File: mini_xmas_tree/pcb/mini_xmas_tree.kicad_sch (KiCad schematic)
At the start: 19 parts, among them J1 Conn_01x02, J2 Conn_01x02, J3 Conn_01x02, J4 Conn_01x02, Q1 BC817, Q2 BC817, Q3 BC817, Q4 BC817

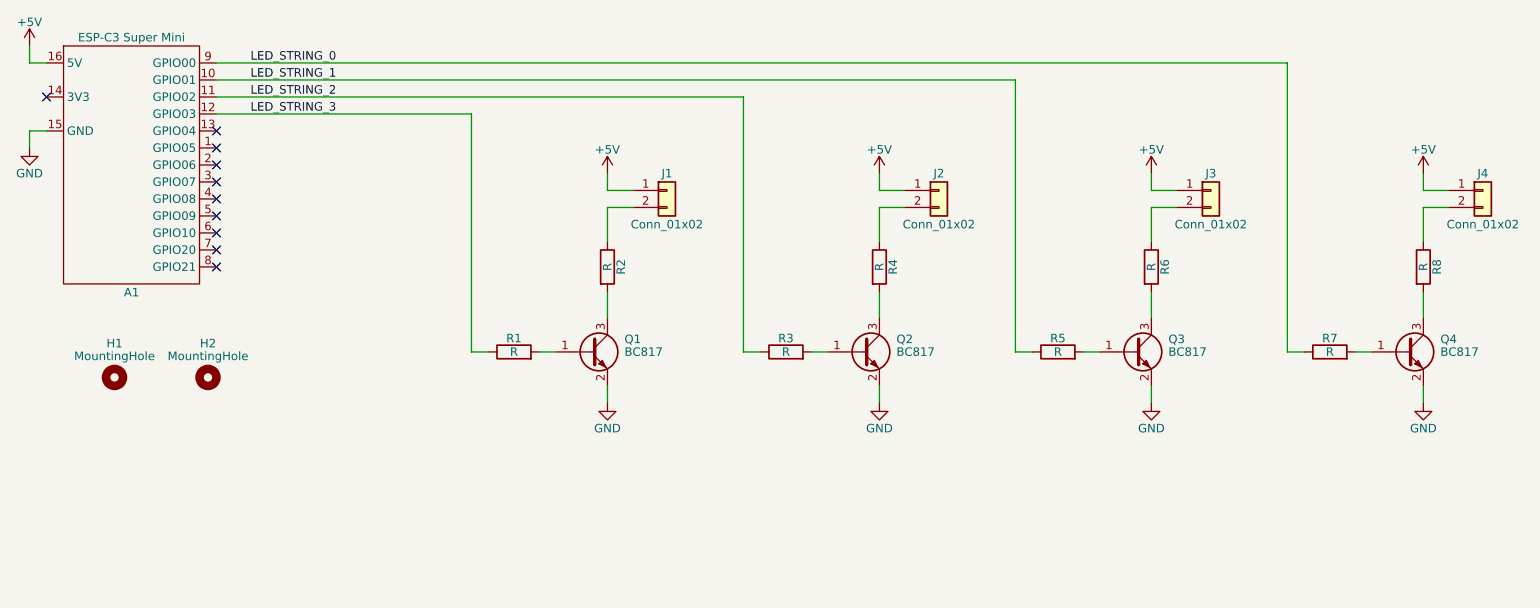
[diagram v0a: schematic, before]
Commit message: create gcode
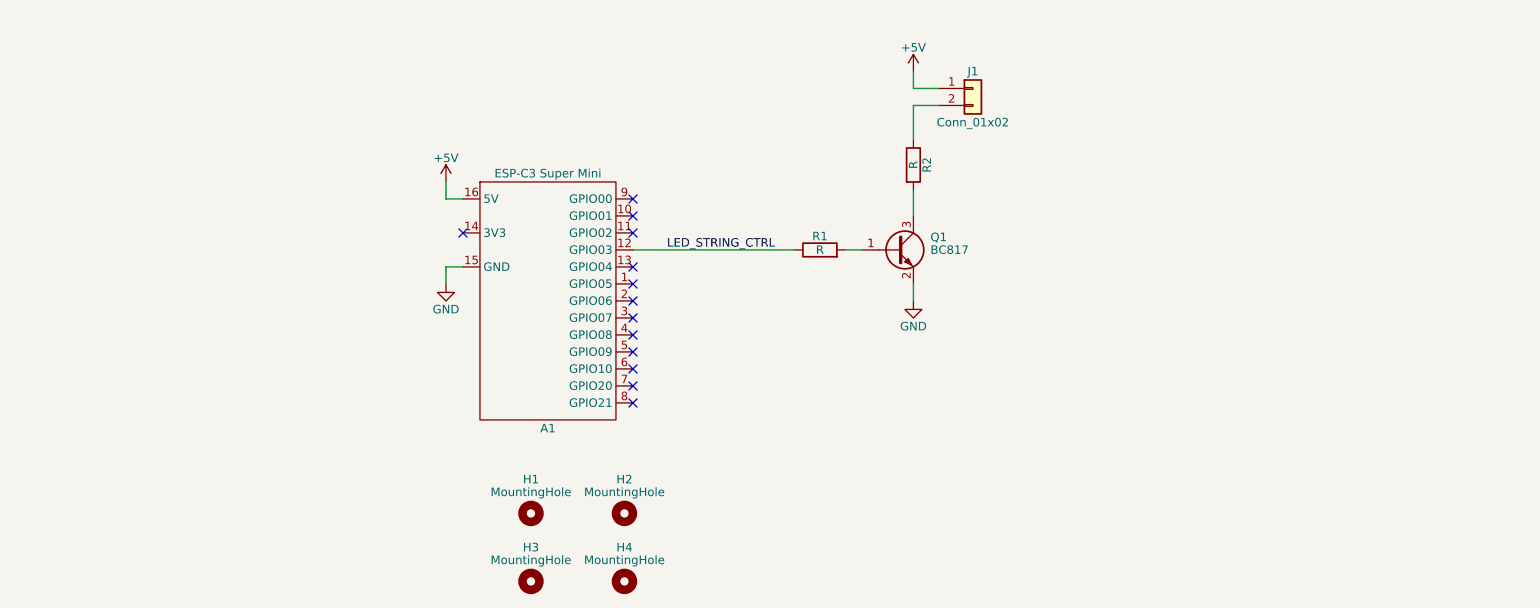
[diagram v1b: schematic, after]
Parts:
- removed J2, J3, J4: Conn_01x02, Connector_PinHeader_2.54mm:PinHeader_1x02_P2.54mm_Vertical, symbol Connector_Generic:Conn_01x02
- removed Q2, Q3, Q4: BC817, Package_TO_SOT_SMD:SOT-23, symbol Transistor_BJT:BC817
- removed R3, R4, R5, R6, R7, R8: R, Resistor_SMD:R_0805_2012Metric_Pad1.20x1.40mm_HandSolder, symbol Device:R
- added H3, H4: MountingHole, MountingHole:MountingHole_3.2mm_M3, symbol Mechanical:MountingHole
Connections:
- net LED_STRING_0: no longer names the net of A1.9 (GPIO00)
- net LED_STRING_1: no longer names the net of A1.10 (GPIO01)
- net LED_STRING_2: no longer names the net of A1.11 (GPIO02)
- net LED_STRING_3 renamed LED_STRING_CTRL
- no-connect marks 10 -> 13
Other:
- moved on the sheet: A1, H1, H2, J1, Q1, R1, R2
